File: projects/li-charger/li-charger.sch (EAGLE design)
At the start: 23 parts, among them J1 Power Jack, Q1 IRF5305, Q2 BC547, Q3 BC327, Q4 BC337, U1 REG1117, U2 Arduino Pro Mini

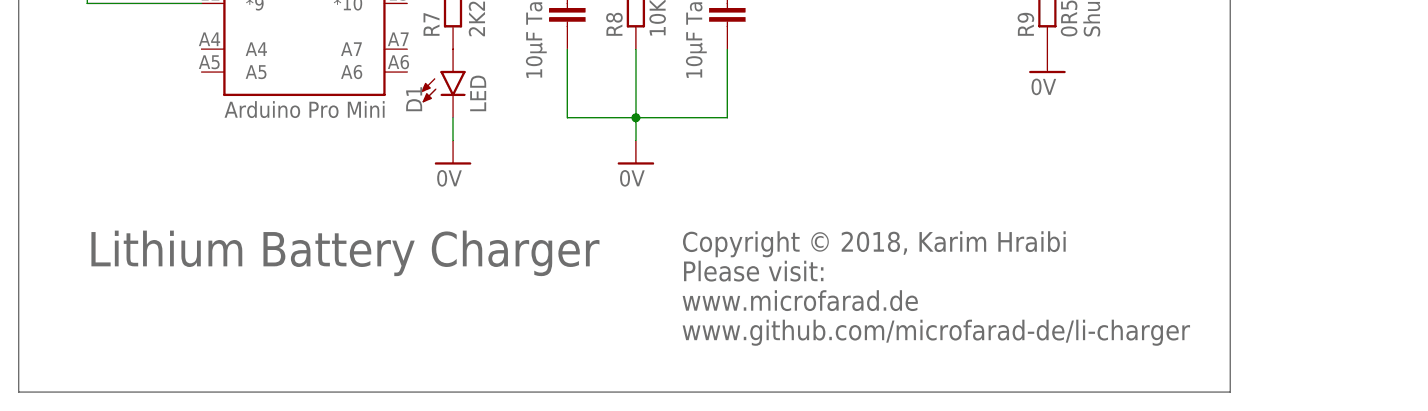
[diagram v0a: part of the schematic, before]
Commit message: Update li-charger.sch
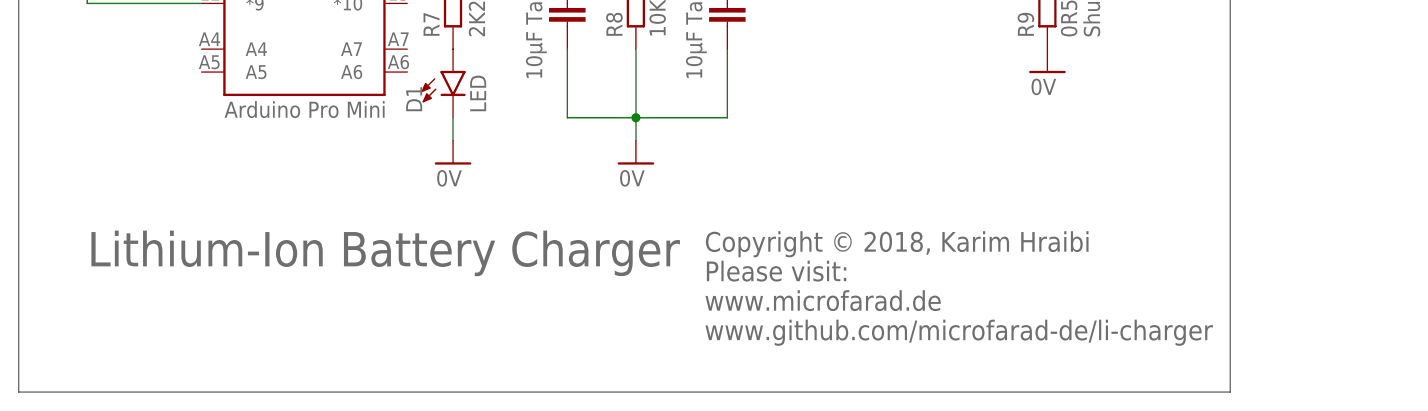
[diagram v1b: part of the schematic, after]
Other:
- note added: "Lithium-Ion Battery Charger"
- note removed: "Lithium Battery Charger"
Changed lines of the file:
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@@
 <wire x1="78.74" y1="-25.4" x2="78.74" y2="104.14" width="0.1524" layer="95"/>
 <wire x1="78.74" y1="104.14" x2="-55.88" y2="104.14" width="0.1524" layer="95"/>
-<text x="-48.26" y="-7.62" size="3.81" layer="95" align="top-left">Lithium Battery Charger</text>
-<text x="17.78" y="-7.62" size="2.1844" layer="95" align="top-left">Copyright © 2018, Karim Hraibi
+<text x="-48.26" y="-7.62" size="3.81" layer="95" align="top-left">Lithium-Ion Battery Charger</text>
+<text x="20.32" y="-7.62" size="2.1844" layer="95" align="top-left">Copyright © 2018, Karim Hraibi
 Please visit:
 www.microfarad.de
